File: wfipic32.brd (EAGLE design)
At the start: 35.5 x 27.6 mm, 34 parts, among them IC1 BMA490L, J1 MLE-105-01-G-DV, J2 MLE-105-01-G-DV, J3 MLE-105-01-G-DV, J4 MLE-105-01-G-DV, U1 PIC32MK0512MCJ048T-I/Y8XTQFP4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, U2 MAX6126B30

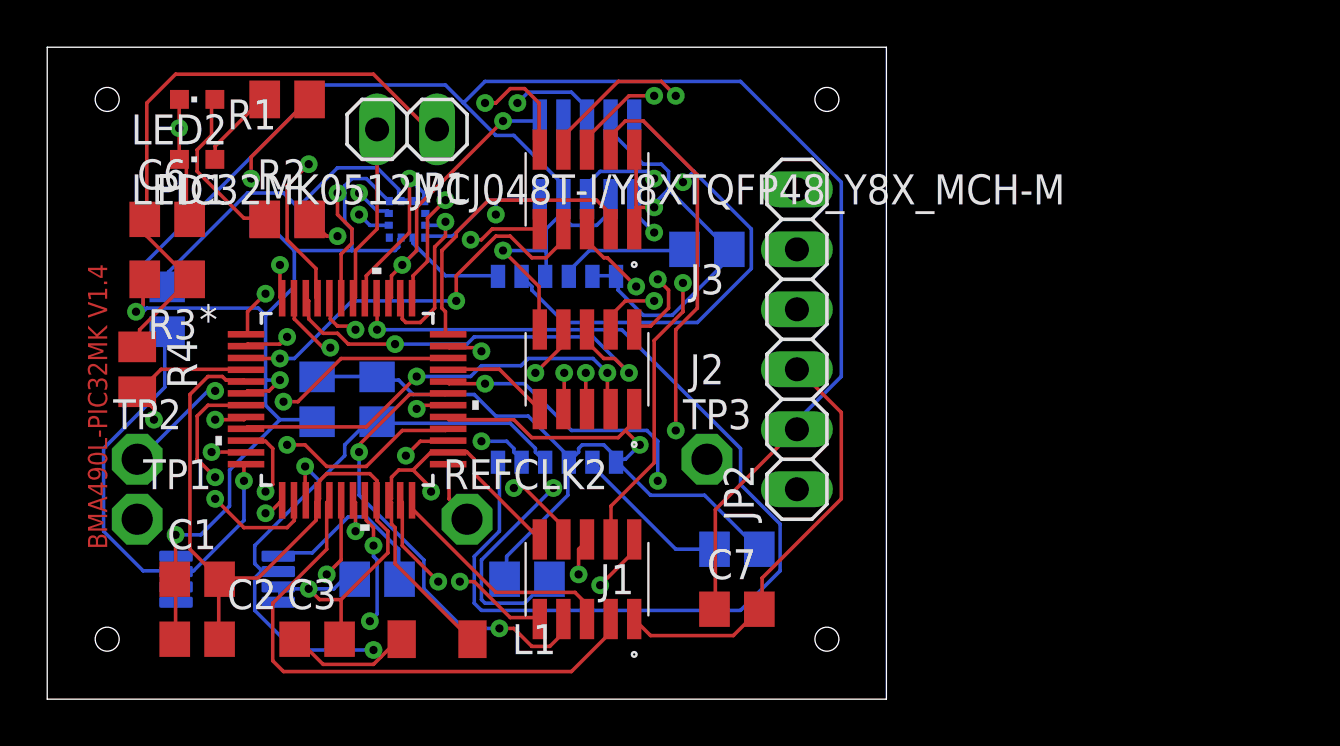
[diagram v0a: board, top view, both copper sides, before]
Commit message: up
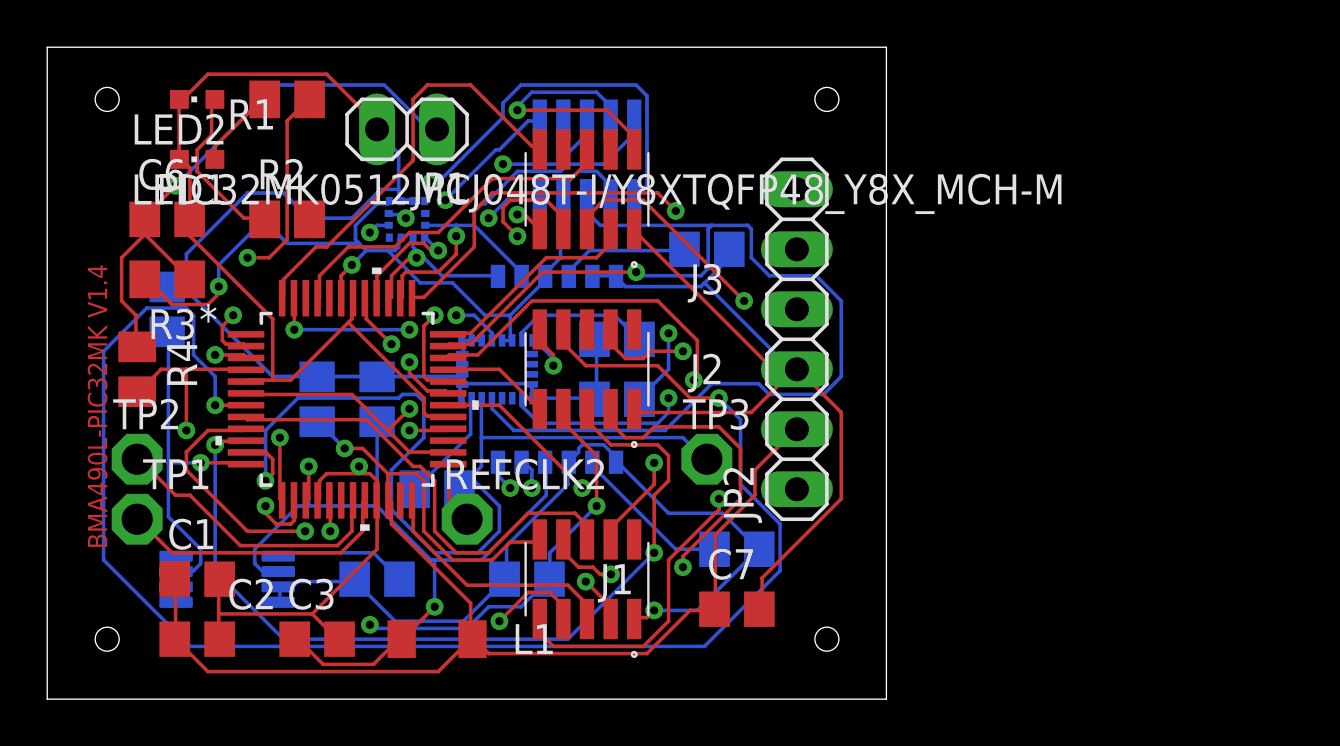
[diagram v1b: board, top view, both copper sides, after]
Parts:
- added C14: 0.1uf, rcl:C0805
- added C15: 0.01uf, rcl:C0805
- added R5: 1k, rcl:M0805
- added U3: LSM9DS1, LSM9DS1:PQFN24P43_350X300X102L35X23N
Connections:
- removed net N$6: TP2.TP, U1.19
- new net N$10: C14.1, U3.24
- new net N$11: C15.1, U3.21
- new net N$12: R5.2, U3.12
- new net N$13: U3.9
- new net TP2: TP2.TP, U1.19, U3.8
- net BMA_INT2: now also R5.1, U3.11
- net EXT_INT2: now also U3.10
- net IMU_CS: now also U3.7
- net SCK2: now also U3.2
- net SDO2: now also U3.4
- net VDD: now also U3.1, U3.22, U3.23, U3.3
- net VSS: now also C14.2, C15.2, U3.13, U3.14, U3.15, U3.16, U3.17, U3.18, U3.19, U3.20, U3.5, U3.6
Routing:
- net EXT_SW2: track 23.5 -> 67.1 mm
- net VSS: track 146.8 -> 186.3 mm, vias 4 -> 3
- net PWM4ER: track 35.3 -> 0.00 mm, vias 2 -> 0
- net PWM4L: track 32.6 -> 0.00 mm, vias 2 -> 0
- net VDD: track 153.1 -> 127.1 mm, vias 6 -> 5
- net EXT_INT2: track 38.0 -> 61.1 mm, vias 3 -> 2
- net AN0: track 18.5 -> 40.4 mm
- net SCK2: track 40.7 -> 19.5 mm, vias 2 -> 1
- net QEA2: track 19.3 -> 0.00 mm, vias 2 -> 0
- net INDX2: track 18.6 -> 0.00 mm, vias 2 -> 0
- net U1RX: track 18.6 -> 0.00 mm, vias 2 -> 0
- net PGD_C1TX: track 51.4 -> 33.8 mm
- net SDI2: track 62.0 -> 44.5 mm, vias 2 -> 3
- net PWM1EN: track 16.2 -> 32.3 mm
- net BMA_INT2: track 50.8 -> 66.8 mm
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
